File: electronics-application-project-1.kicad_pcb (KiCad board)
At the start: 2 copper layers, 52 x 32.5 mm, 42 parts, among them J1 Conn_02x03_Odd_Even, U1 W5500, U2 ARJM11C7-114-BA-EW2, U3 LM2574-3.3YN, U4 ATTINY85-20SU, Y2 ABLS7M2-25.000MHZ-D-2Y-T

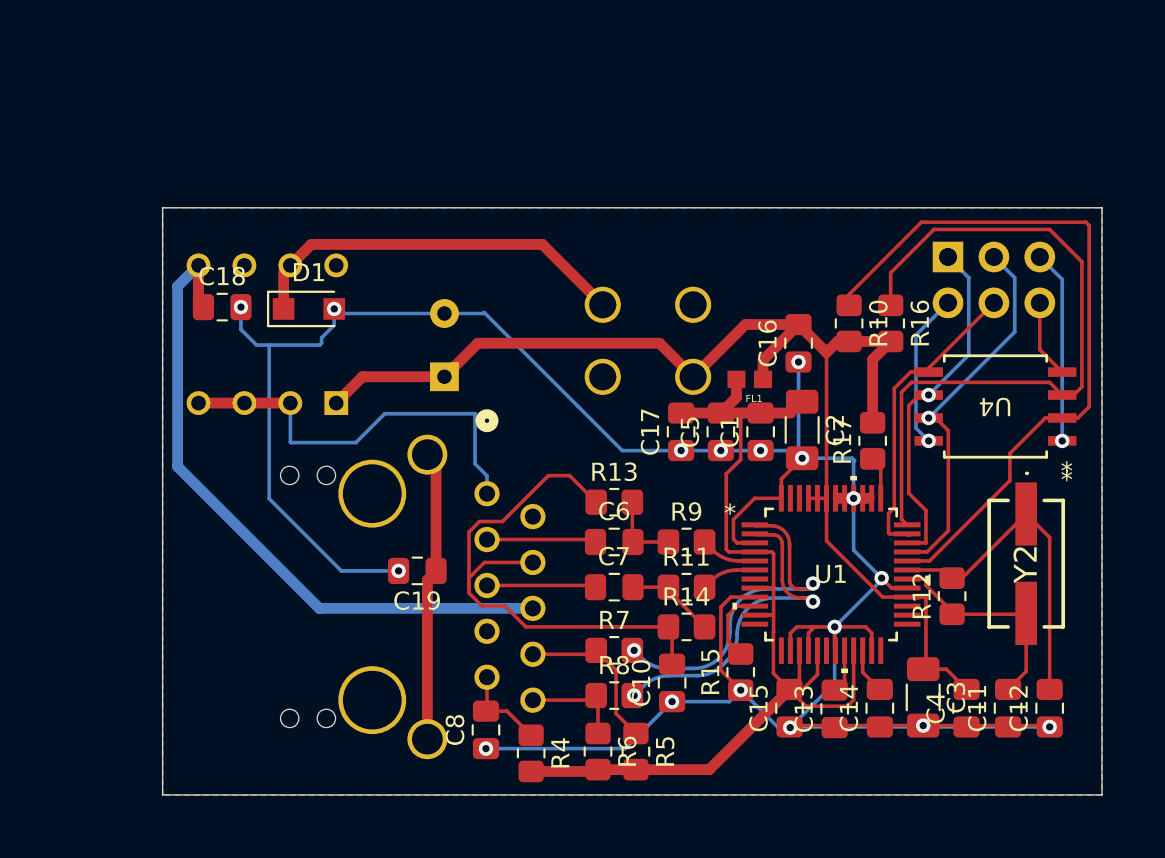
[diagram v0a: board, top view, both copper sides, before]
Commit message: v2
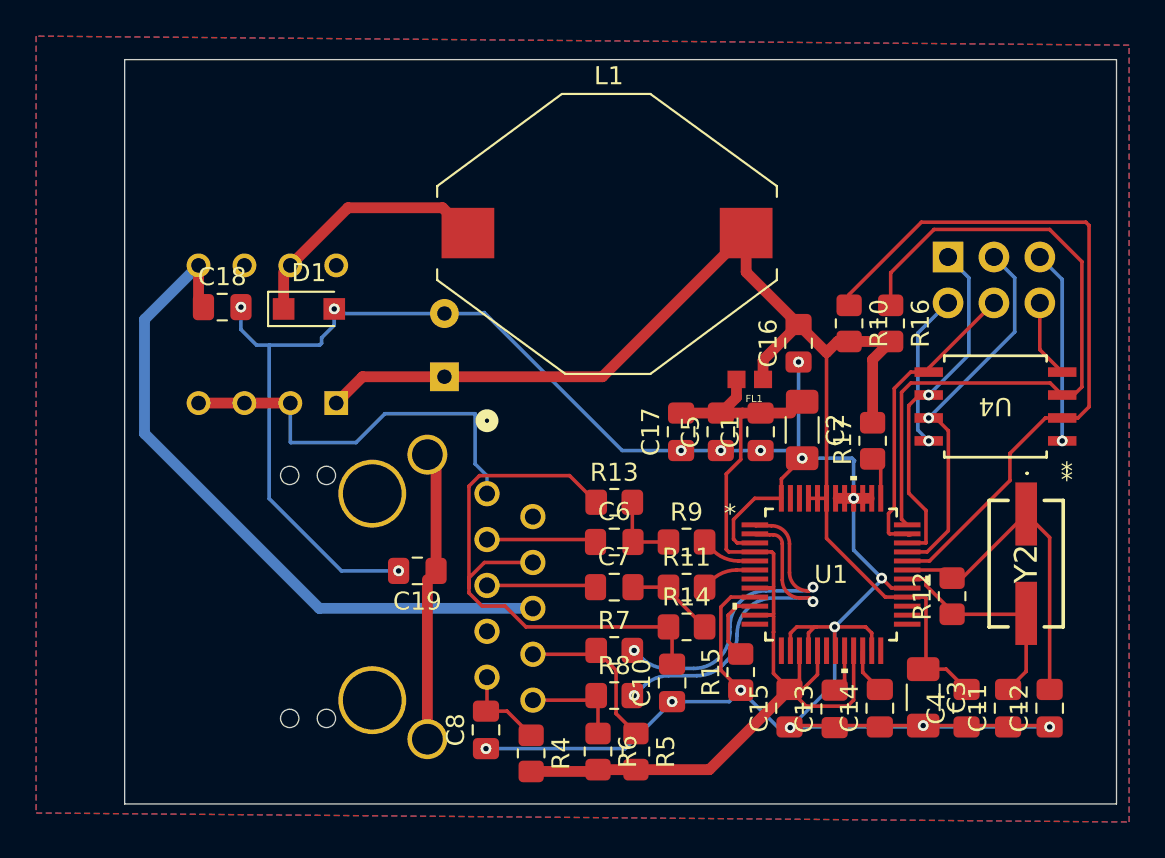
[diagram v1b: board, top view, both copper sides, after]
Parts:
- L1: value 12LRS334C -> 330uH; footprint Imported:IND_MURATA_1200LRS_MUR -> Inductor_SMD:L_Wuerth_WE-PD4-Typ-X; moved to F.Cu
- moved L1 10.1 mm to (134.1, 72.4), turned to 0 degrees
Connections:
- L1 pad 2: unconnected-(L1-NC-Pad2) -> 3.3V_D
- U2 pad 1: GND -> Net-(U2-VC2-)
- U3 pad 2: GND -> Net-(U2-VC2-)
- U3 pad 3: GND -> Net-(U2-VC2-)
- U3 pad 4: GND -> Net-(U2-VC2-)
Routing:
- net GND: track 180.0 -> 157.2 mm
- net Net-(U2-VC2-): track 0.00 -> 22.8 mm
- net Net-(D1-K): track 21.7 -> 14.3 mm
- net 3.3V_D: track 68.8 -> 72.6 mm
- net Net-(U2-VC2+): track 37.0 -> 38.5 mm
- net Net-(U2-RCT): track 31.2 -> 32.3 mm
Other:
- board size 52 x 32.5 mm -> 54.9 x 41.2 mm
